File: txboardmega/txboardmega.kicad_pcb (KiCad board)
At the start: 2 copper layers, 86.4 x 87.6 mm, 27 parts, among them J1 Power, J10 Switch 2, J11 Switch 3, J12 Switch 4, J13 Switch 5, J14 Switch 6, J15 Encoder, J16 TX Module, J2 Display, J3 Analog 1, J4 Analog 2, J5 Analog 3, J6 Analog 4, J7 Analog 5, J8 Analog 6, J9 Switch 1, U1 ARD_Mega2560_pro, U2 LM7809_TO220

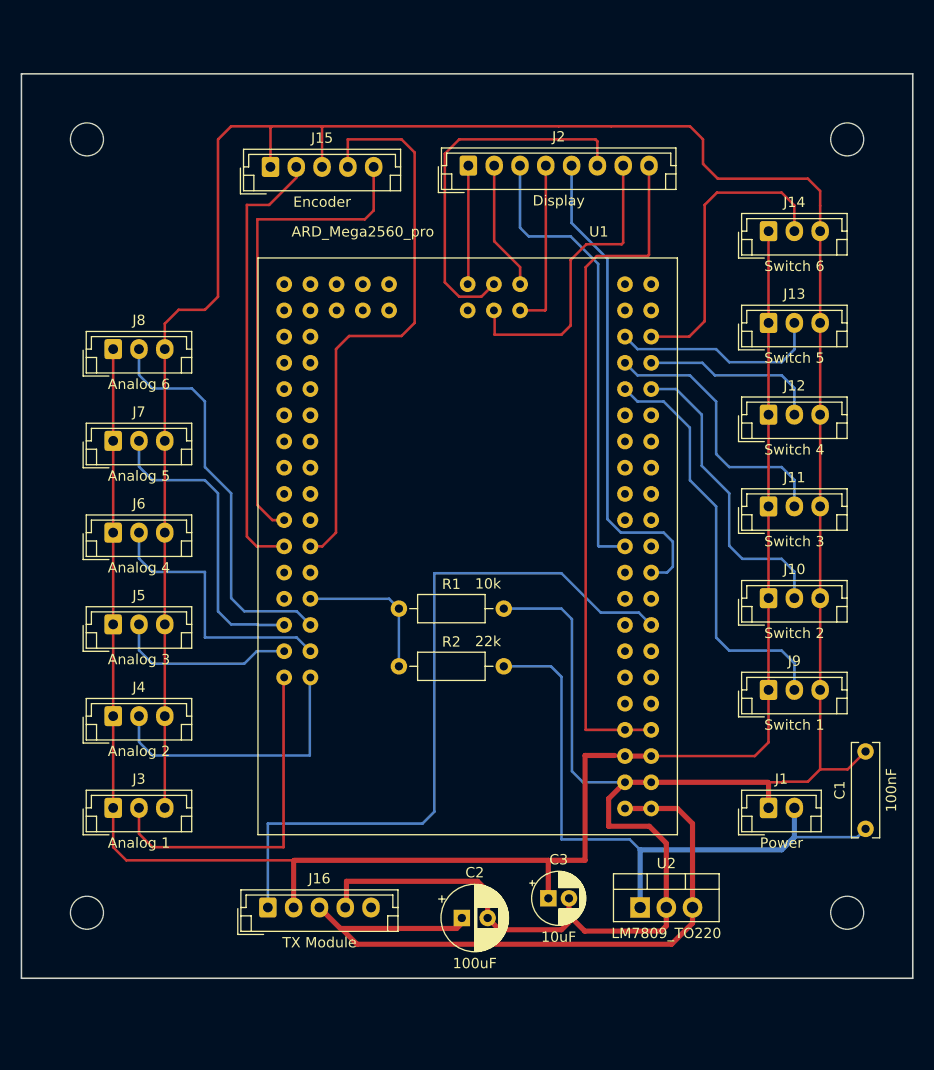
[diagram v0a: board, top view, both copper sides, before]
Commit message: Board for Robbe Supra
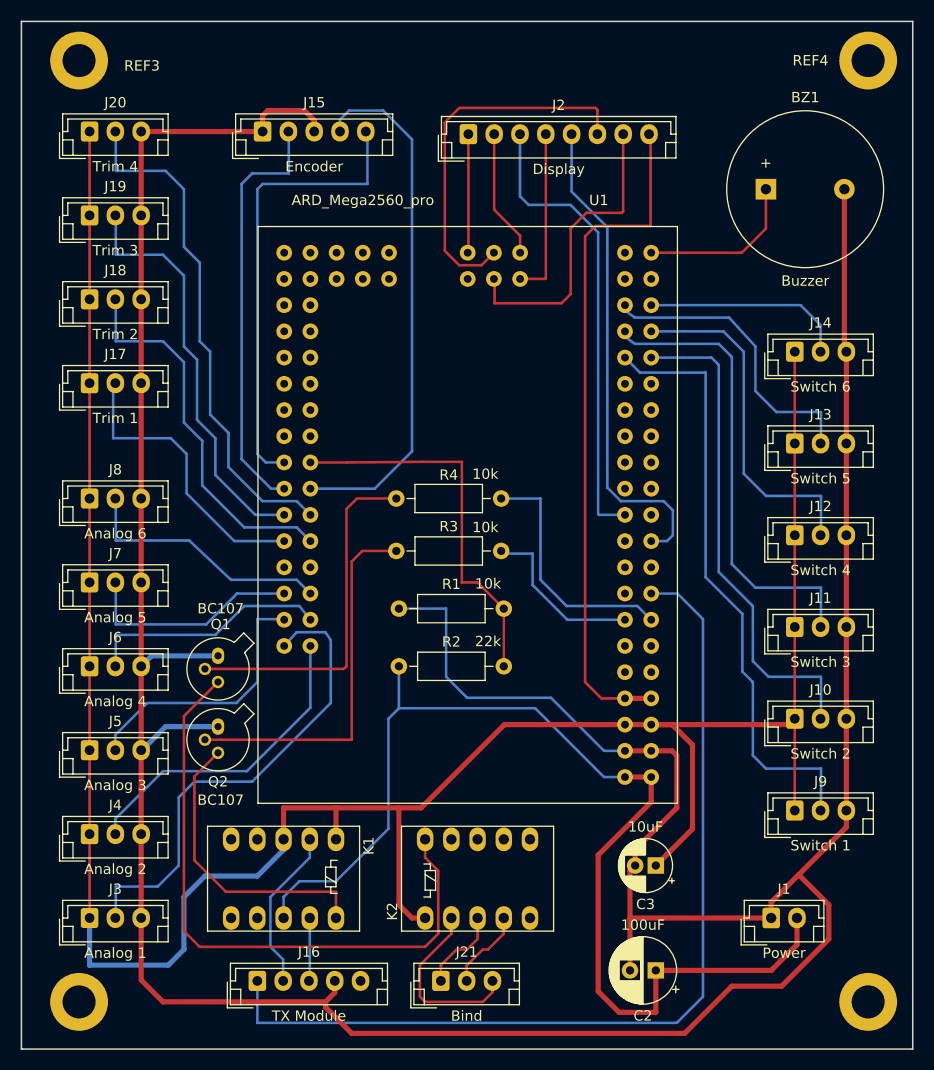
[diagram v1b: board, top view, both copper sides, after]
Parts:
- removed C1: 100nF, Capacitor_THT:C_Rect_L9.0mm_W2.5mm_P7.50mm_MKT
- removed REF** (x4): MountingHole_3.2mm_M3_DIN965, MountingHole:MountingHole_3.2mm_M3_DIN965
- removed U2: LM7809_TO220, Package_TO_SOT_THT:TO-220-3_Vertical
- added BZ1: Buzzer, Buzzer_Beeper:Buzzer_15x7.5RM7.6, F.Cu at (166.1, 79.8)
- added J17: Trim 1, Connector_JST:JST_EH_B3B-EH-A_1x03_P2.50mm_Vertical, F.Cu at (100.6, 98.6)
- added J18: Trim 2, Connector_JST:JST_EH_B3B-EH-A_1x03_P2.50mm_Vertical, F.Cu at (100.6, 90.4)
- added J19: Trim 3, Connector_JST:JST_EH_B3B-EH-A_1x03_P2.50mm_Vertical, F.Cu at (100.6, 82.3)
- added J20: Trim 4, Connector_JST:JST_EH_B3B-EH-A_1x03_P2.50mm_Vertical, F.Cu at (100.6, 74.2)
- added J21: Bind, Connector_JST:JST_EH_B3B-EH-A_1x03_P2.50mm_Vertical, F.Cu at (134.6, 156.5)
- added K1: HF on, Relay_THT:Relay_DPDT_FRT5, F.Cu at (124.5, 142.7)
- added K2: Bind, Relay_THT:Relay_DPDT_FRT5, F.Cu at (133.1, 150.4)
- added Q1: BC107, Package_TO_SOT_THT:TO-18-3, F.Cu at (113.0, 125.0)
- added Q2: BC107, Package_TO_SOT_THT:TO-18-3, F.Cu at (113.0, 131.8)
- added R3: 10k, Resistor_THT:R_Axial_DIN0207_L6.3mm_D2.5mm_P10.16mm_Horizontal, F.Cu at (130.3, 114.8)
- added R4: 10k, Resistor_THT:R_Axial_DIN0207_L6.3mm_D2.5mm_P10.16mm_Horizontal, F.Cu at (140.5, 109.7)
- added REF1: MountingHole_3.2mm_M3_DIN965_Pad, MountingHole:MountingHole_3.2mm_M3_DIN965_Pad, F.Cu at (176.0, 158.5)
- added REF2: MountingHole_3.2mm_M3_DIN965_Pad, MountingHole:MountingHole_3.2mm_M3_DIN965_Pad, F.Cu at (99.6, 158.5)
- added REF3: MountingHole_3.2mm_M3_DIN965_Pad, MountingHole:MountingHole_3.2mm_M3_DIN965_Pad, F.Cu at (99.6, 67.3)
- added REF4: MountingHole_3.2mm_M3_DIN965_Pad, MountingHole:MountingHole_3.2mm_M3_DIN965_Pad, F.Cu at (176.0, 67.3)
- moved C2 19.5 mm to (155.4, 155.4), turned to 180 degrees
- moved J8 14.7 mm to (100.6, 109.7)
- moved J7 13.9 mm to (100.6, 117.9)
- moved J6 13.2 mm to (100.6, 126.0)
- moved J5 12.4 mm to (100.6, 134.1)
- moved J11 12.0 mm to (168.9, 122.2)
- moved J12 12.0 mm to (168.9, 113.3)
- moved J13 12.0 mm to (168.9, 104.4)
- moved J14 12.0 mm to (168.9, 95.5)
- moved J10 12.0 mm to (168.9, 131.1)
- moved J9 12.0 mm to (168.9, 140.0)
- moved J4 11.7 mm to (100.6, 142.2)
- moved J3 10.9 mm to (100.6, 150.4)
- moved C3 10.9 mm to (155.4, 145.3), turned to 180 degrees
- moved J1 10.7 mm to (166.6, 150.4)
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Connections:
- C2 pad 2: Net-(C1-Pad2) -> Net-(BZ1-Pad2)
- C3 pad 2: Net-(C1-Pad2) -> Net-(BZ1-Pad2)
- J1 pad 1: Net-(C1-Pad2) -> Net-(BZ1-Pad2)
- J1 pad 2: Net-(C1-Pad1) -> Net-(C2-Pad1)
- J10 pad 3: Net-(C1-Pad2) -> Net-(BZ1-Pad2)
- J11 pad 3: Net-(C1-Pad2) -> Net-(BZ1-Pad2)
- J12 pad 3: Net-(C1-Pad2) -> Net-(BZ1-Pad2)
- J13 pad 3: Net-(C1-Pad2) -> Net-(BZ1-Pad2)
- J14 pad 3: Net-(C1-Pad2) -> Net-(BZ1-Pad2)
- J15 pad 1: Net-(C1-Pad2) -> Net-(BZ1-Pad2)
- J15 pad 3: Net-(C1-Pad2) -> Net-(BZ1-Pad2)
- J16 pad 2: Net-(C3-Pad1) -> Net-(J16-Pad2)
- J16 pad 3: Net-(C2-Pad1) -> Net-(J16-Pad3)
- J16 pad 4: Net-(C1-Pad2) -> Net-(BZ1-Pad2)
- J3 pad 3: Net-(C1-Pad2) -> Net-(BZ1-Pad2)
- J4 pad 3: Net-(C1-Pad2) -> Net-(BZ1-Pad2)
- J5 pad 3: Net-(C1-Pad2) -> Net-(BZ1-Pad2)
- J6 pad 3: Net-(C1-Pad2) -> Net-(BZ1-Pad2)
- J7 pad 3: Net-(C1-Pad2) -> Net-(BZ1-Pad2)
- J8 pad 3: Net-(C1-Pad2) -> Net-(BZ1-Pad2)
- J9 pad 3: Net-(C1-Pad2) -> Net-(BZ1-Pad2)
- R1 pad 1: Net-(R1-Pad1) -> Net-(BZ1-Pad2)
- R1 pad 2: Net-(C1-Pad2) -> Net-(R1-Pad2)
- R2 pad 1: Net-(R1-Pad1) -> Net-(C2-Pad1)
- R2 pad 2: Net-(C1-Pad1) -> Net-(R1-Pad2)
- U1 pad 3: Net-(C1-Pad2) -> Net-(BZ1-Pad2)
- U1 pad 4: Net-(C1-Pad2) -> Net-(BZ1-Pad2)
- U1 pad 50: Net-(R1-Pad1) -> Net-(U1-Pad50)
- U1 pad 53: Net-(J15-Pad2) -> Net-(J19-Pad2)
- U1 pad 54: Net-(J15-Pad4) -> Net-(J20-Pad2)
- U1 pad 55: Net-(J15-Pad5) -> Net-(J15-Pad2)
- U1 pad 56: Net-(U1-Pad56) -> Net-(J15-Pad4)
- U1 pad 57: Net-(U1-Pad57) -> Net-(J15-Pad5)
- U1 pad 58: Net-(U1-Pad58) -> Net-(R1-Pad2)
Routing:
- net Net-(BZ1-Pad2): track 0.00 -> 348.4 mm
- net Net-(C1-Pad2): track 309.3 -> 0.00 mm
- net Net-(C3-Pad1): track 180.8 -> 243.3 mm
- net Net-(C1-Pad1): track 61.1 -> 0.00 mm
- net Net-(K2-Pad10): track 0.00 -> 61.0 mm
- net Net-(J20-Pad2): track 0.00 -> 49.7 mm
- net Net-(C2-Pad1): track 67.8 -> 109.0 mm
- net Net-(J19-Pad2): track 0.00 -> 40.1 mm
- net Net-(R1-Pad2): track 0.00 -> 37.1 mm
- net Net-(J18-Pad2): track 0.00 -> 36.9 mm
- net Net-(Q2-Pad2): track 0.00 -> 36.2 mm
- net Net-(Q1-Pad2): track 0.00 -> 34.3 mm
- net Net-(K1-Pad10): track 0.00 -> 28.9 mm
- net Net-(J17-Pad2): track 0.00 -> 28.4 mm
- net Net-(R4-Pad1): track 0.00 -> 24.0 mm
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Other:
- board size 86.4 x 87.6 mm -> 86.4 x 99.6 mm
